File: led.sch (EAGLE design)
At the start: 4 parts

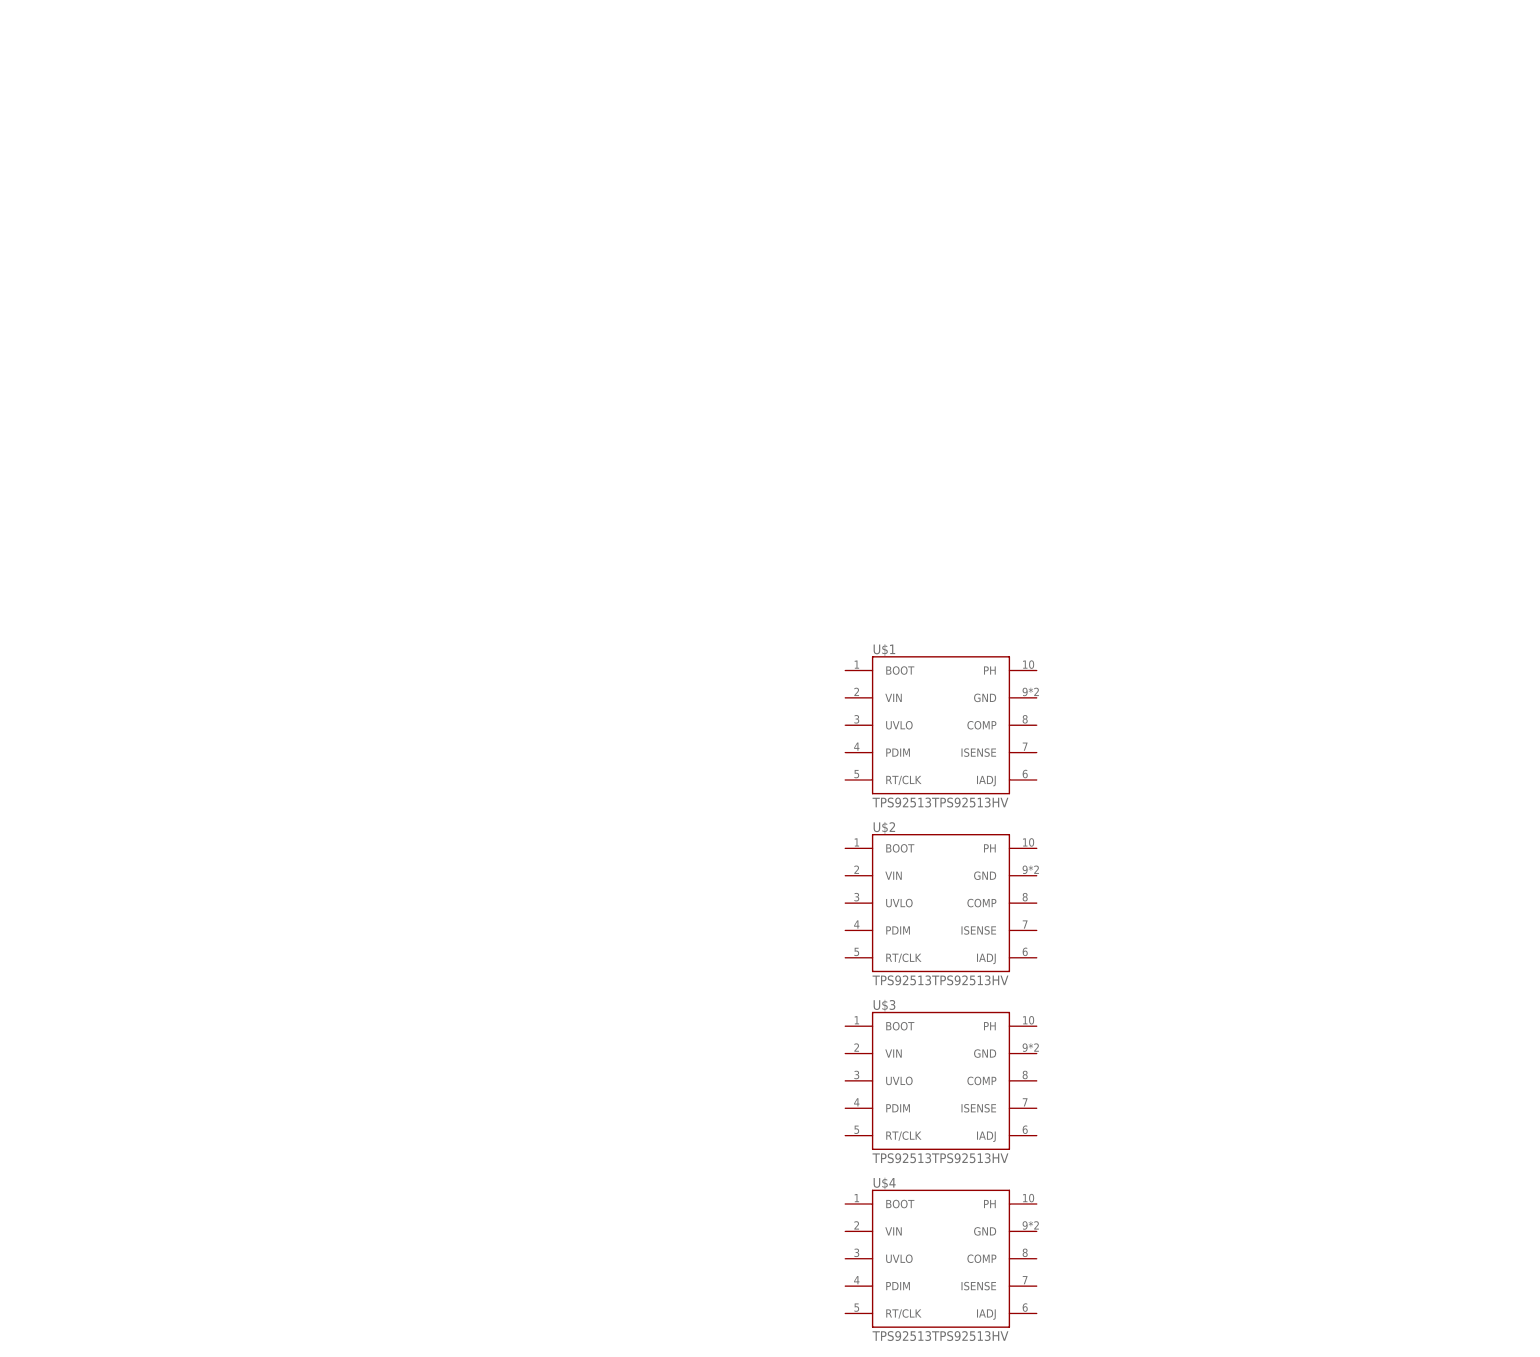
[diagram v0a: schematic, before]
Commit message: save
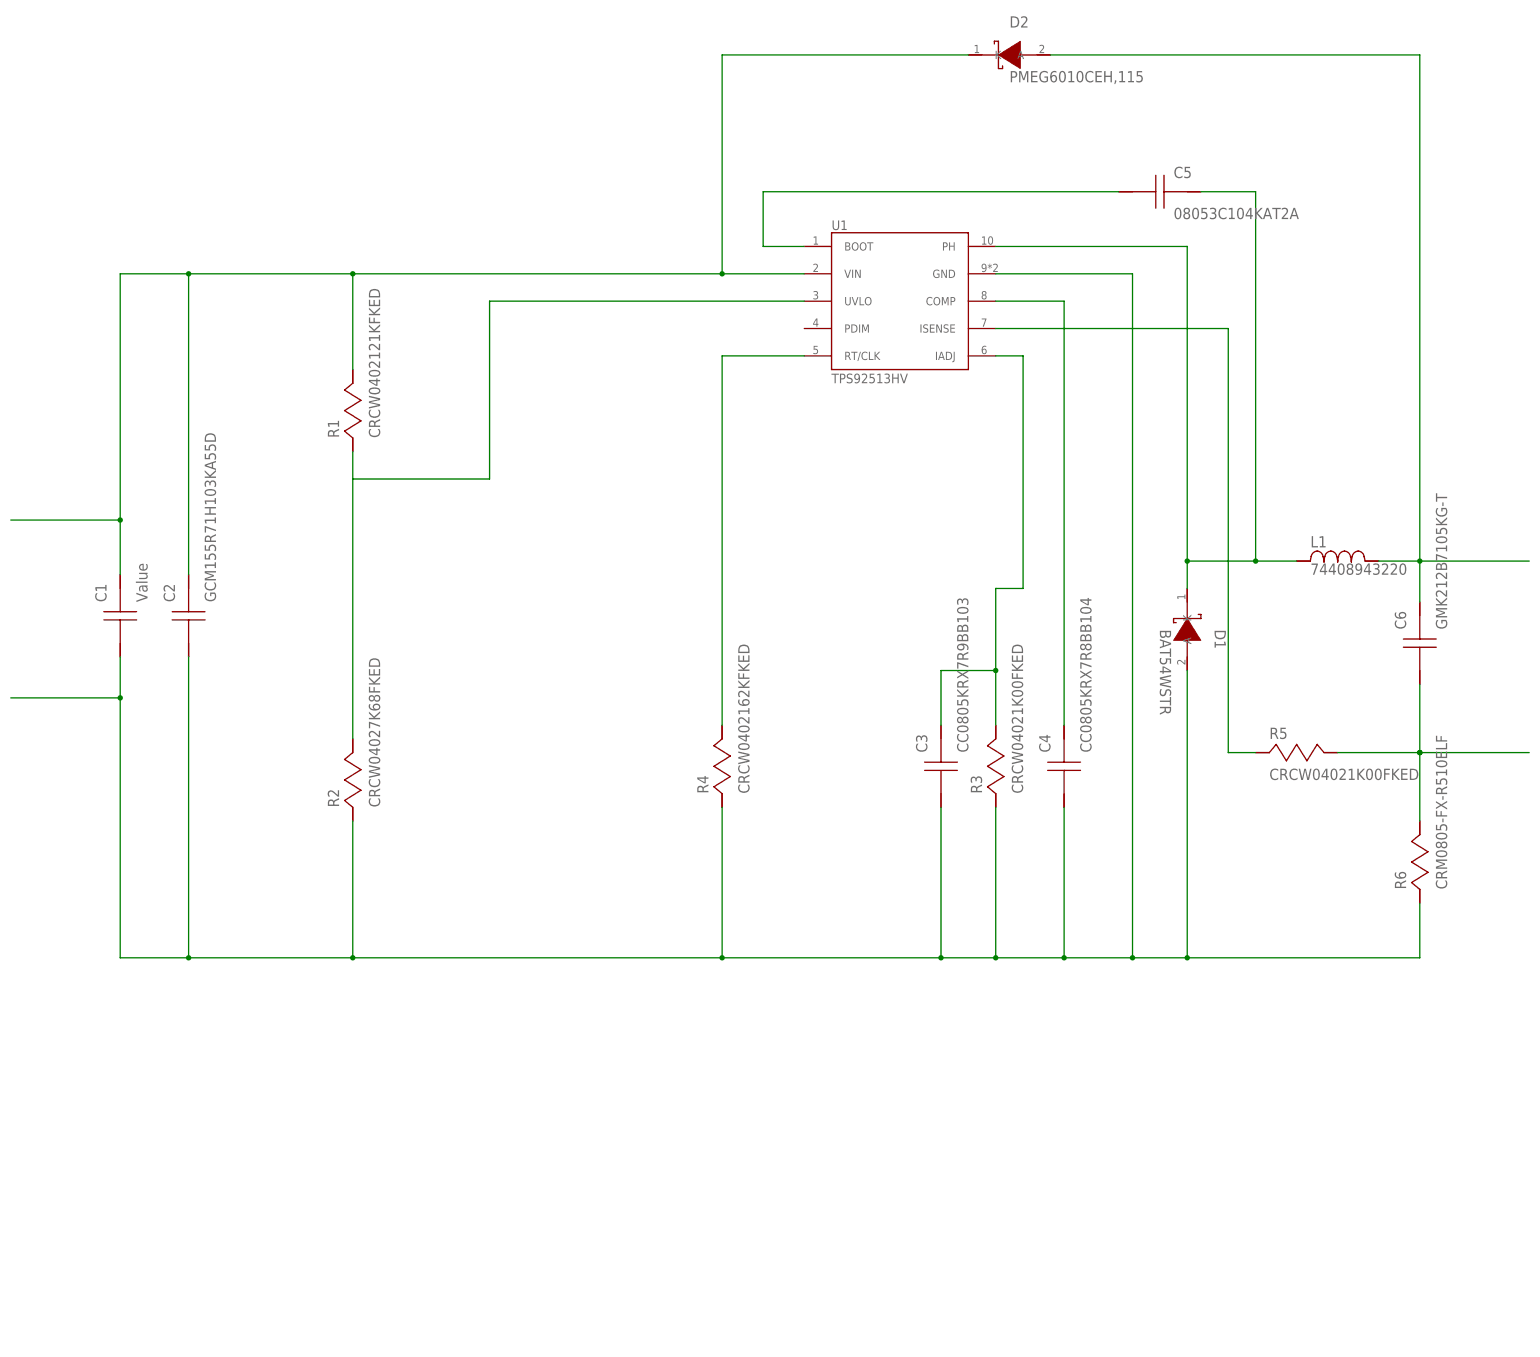
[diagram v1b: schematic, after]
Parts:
- removed U$1, U$2, U$3, U$4: TPS92513TPS92513HV, derek:TPS92513TPS92513HV
- added C1: Value, derek:GRM32ER71J106KA12L
- added C2: GCM155R71H103KA55D, derek:GCM155R71H103KA55D
- added C3: CC0805KRX7R9BB103, derek:CC0805KRX7R9BB103
- added C4: CC0805KRX7R8BB104, derek:CC0805KRX7R8BB104
- added C5: 08053C104KAT2A, derek:08053C104KAT2A
- added C6: GMK212B7105KG-T, derek:GMK212B7105KG-T
- added D1: BAT54WSTR, derek:BAT54WSTR
- added D2: PMEG6010CEH,115, derek:PMEG6010CEH,115
- added L1: 74408943220, derek:74408943220
- added R1: CRCW0402121KFKED, derek:CRCW0402121KFKED
- added R2: CRCW04027K68FKED, derek:CRCW04027K68FKED
- added R3, R5: CRCW04021K00FKED, derek:CRCW04021K00FKED
- added R4: CRCW0402162KFKED, derek:CRCW0402162KFKED
- added R6: CRM0805-FX-R510ELF, derek:CRM0805-FX-R510ELF
- added U1: TPS92513HV, derek:TPS92513HV
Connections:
- new net N$1: C1.2, C2.2, C3.2, C4.2, D1.A, R2.2, R3.2, R4.2, R6.2, U1.GND
- new net N$10: C5.2, U1.BOOT
- new net N$11: R5.2, U1.ISENSE
- new net N$2: C3.1, R3.1, U1.IADJ
- new net N$3: R1.2, R2.1, U1.UVLO
- new net N$4: C1.1, C2.1, D2.K, R1.1, U1.VIN
- new net N$5: C5.1, D1.K, L1.1, U1.PH
- new net N$6: C6.2, R5.1, R6.1
- new net N$7: C6.1, D2.A, L1.2
- new net N$8: R4.1, U1.RT/CLK
- new net N$9: C4.1, U1.COMP
